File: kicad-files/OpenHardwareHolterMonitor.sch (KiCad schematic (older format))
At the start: 30 parts, among them CON1 Micro_SD_Card, J1 Conn_02x06_Odd_Even, P1 Custom_FTDI, Q1 S8050, Q2 S8050, Q3 Q_NMOS_DGS, Q4 Q_NMOS_DGS, U1 ESP-WROOM-32, Y1 32768Hz

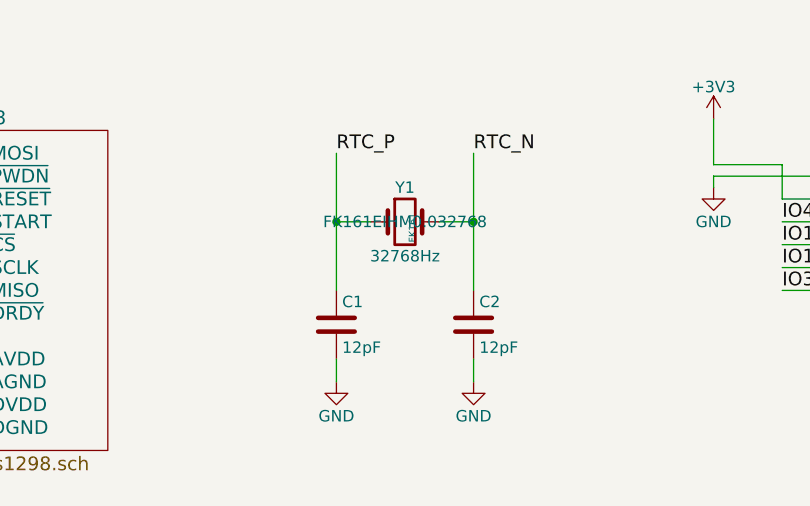
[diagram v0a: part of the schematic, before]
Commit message: add the first few part numbers
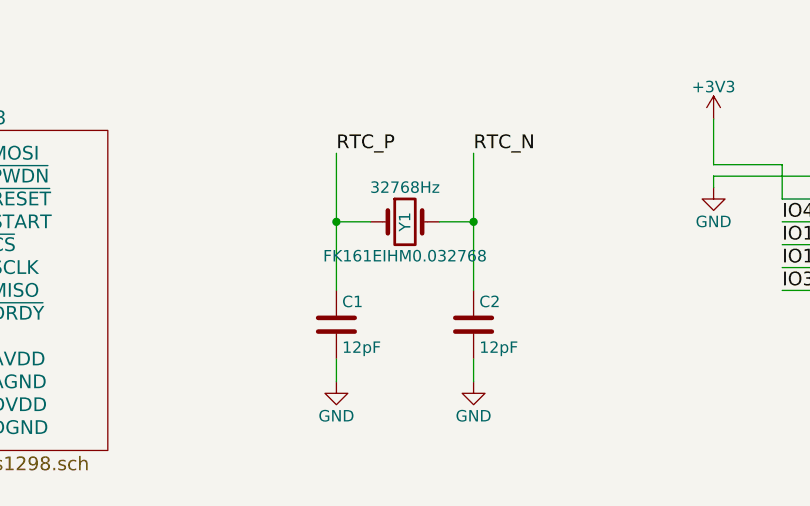
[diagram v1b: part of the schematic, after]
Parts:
- C1, C2: manufacturer-pn (none) -> C0603C120J5GAC
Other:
- note removed: "FK161"
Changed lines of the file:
@@
 U 1 1 5AB80CB4
 P 8250 2300
-F 0 "Y1" H 8250 2450 50  0000 C CNN
-F 1 "32768Hz" H 8250 2150 50  0000 C CNN
+F 0 "Y1" V 8250 2300 50  0000 C CNN
+F 1 "32768Hz" H 8250 2450 50  0000 C CNN
 F 2 "crystals:K161" H 8250 2300 50  0001 C CNN
 F 3 "" H 8250 2300 50  0000 C CNN
-F 4 "FK161EIHM0.032768" H 8250 2300 50  0000 C CNN "manufacturer-pn"
+F 4 "FK161EIHM0.032768" H 8250 2150 50  0000 C CNN "manufacturer-pn"
 	1    8250 2300
 	1    0    0    -1
@@
 F 2 "Capacitors_SMD:C_0603_HandSoldering" H 7988 2600 50  0001 C CNN
 F 3 "" H 7950 2750 50  0000 C CNN
+F 4 "C0603C120J5GAC" H 0   0   50  0001 C CNN "manufacturer-pn"
 	1    7950 2750
 	1    0    0    -1
@@
 F 2 "Capacitors_SMD:C_0603_HandSoldering" H 8588 2600 50  0001 C CNN
 F 3 "" H 8550 2750 50  0000 C CNN
+F 4 "C0603C120J5GAC" H 0   0   50  0001 C CNN "manufacturer-pn"
 	1    8550 2750
 	1    0    0    -1
@@
 Text Label 8550 2000 0    60   ~ 0
 RTC_N
-Text Notes 8300 2400 1    30   ~ 0
-FK161
 Wire Wire Line
 	1400 2200 1100 2200
